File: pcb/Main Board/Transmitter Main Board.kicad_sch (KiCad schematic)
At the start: 16 parts, among them J1 Battery, J10 Neopixel Out, J2 BATTERY MONITOR, J3 i2c, J4 XY JOYSTICK, J5 VR3, J6 Steering, J7 Throttle, J8 UART6/i2c2, J9 UART7, U1 Teensy4.1, U2 TLV73312PDBV, U3 NRF24L01_Breakout

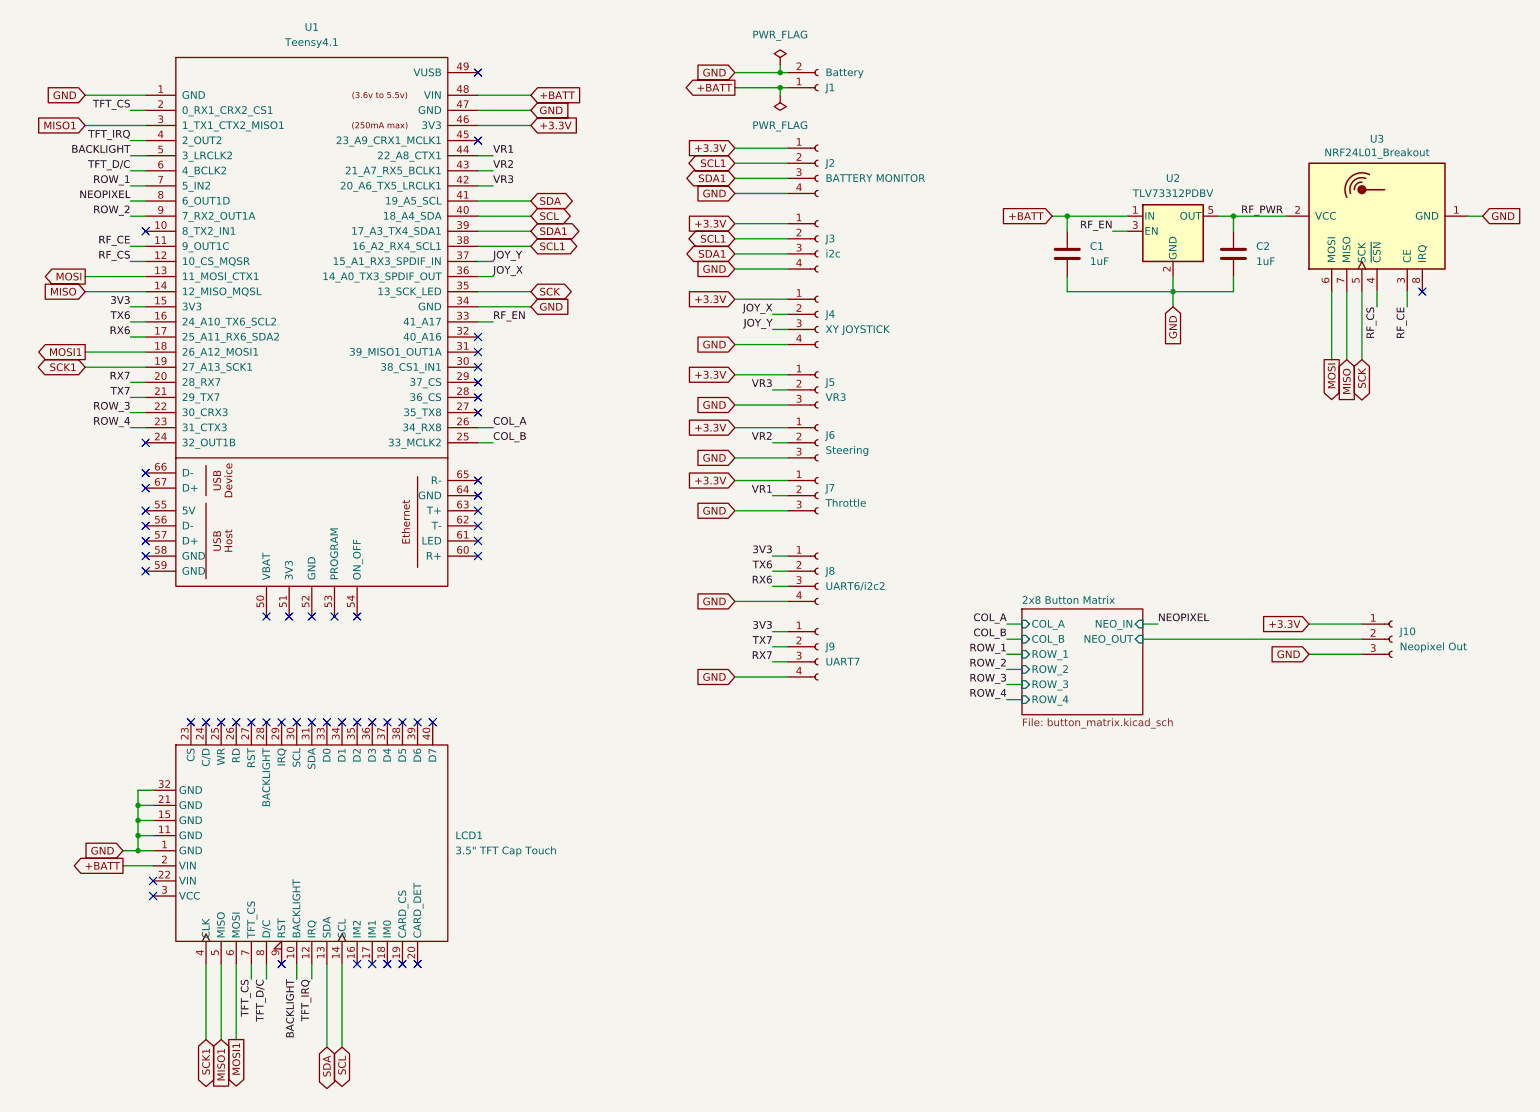
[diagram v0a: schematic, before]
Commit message: Final final routing
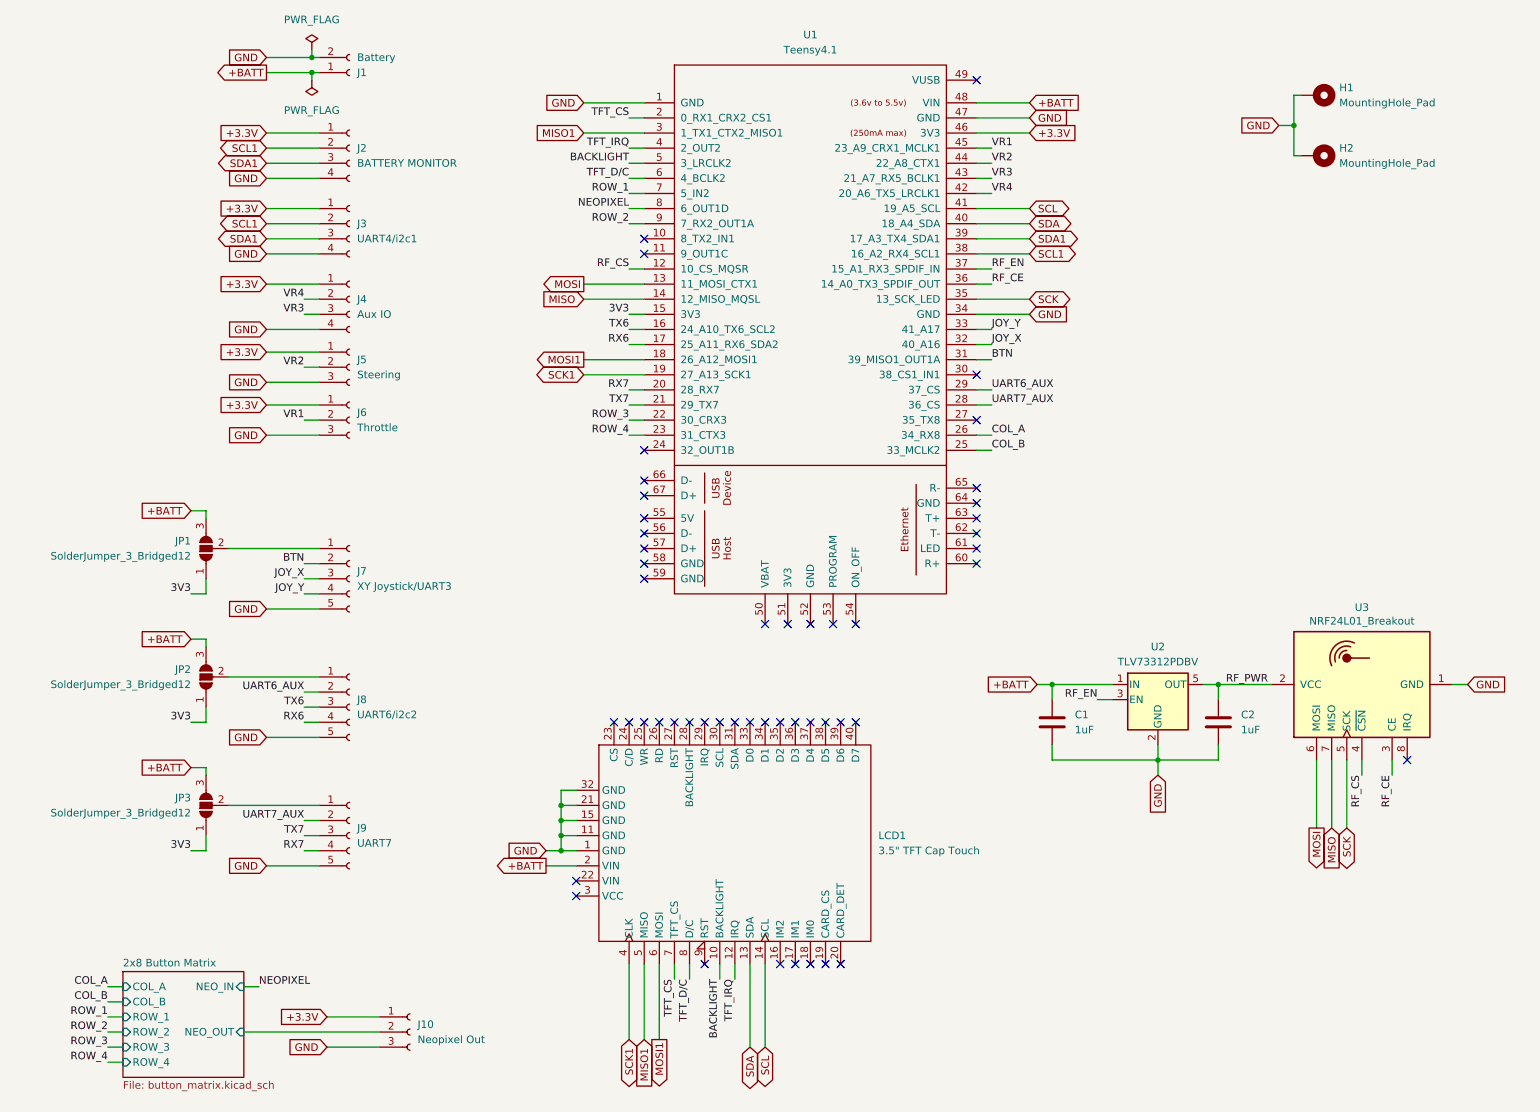
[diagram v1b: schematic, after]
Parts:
- added H1, H2: MountingHole_Pad, MountingHole:MountingHole_3.2mm_M3_Pad, symbol Mechanical:MountingHole_Pad
- added JP1, JP2, JP3: SolderJumper_3_Bridged12, Jumper:SolderJumper-3_P2.0mm_Open_TrianglePad1.0x1.5mm, symbol Jumper:SolderJumper_3_Open
- J3: value i2c -> UART4/i2c1
- J4: renamed from J5; value VR3 -> Aux IO; footprint Connector_JST:JST_PH_B3B-PH-K_1x03_P2.00mm_Vertical -> Connector_JST:JST_PH_B4B-PH-K_1x04_P2.00mm_Vertical; symbol Connector:Conn_01x03_Socket -> Connector:Conn_01x04_Socket
- J7: renamed from J4; value XY JOYSTICK -> XY Joystick/UART3; footprint Connector_JST:JST_PH_B4B-PH-K_1x04_P2.00mm_Vertical -> Connector_JST:JST_PH_B5B-PH-K_1x05_P2.00mm_Vertical; symbol Connector:Conn_01x04_Socket -> Connector:Conn_01x05_Socket
- J8, J9: footprint Connector_JST:JST_PH_B4B-PH-K_1x04_P2.00mm_Vertical -> Connector_JST:JST_PH_B5B-PH-K_1x05_P2.00mm_Vertical; symbol Connector:Conn_01x04_Socket -> Connector:Conn_01x05_Socket
- renumbered J6 to J5, J7 to J6
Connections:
- net +3.3V: no longer J7.1 (Pin_1)
- net +BATT: now also JP1.3 (B), JP2.3 (B), JP3.3 (B)
- net 3V3: now also JP1.1 (A), JP2.1 (A), JP3.1 (A); no longer J8.1 (Pin_1), J9.1 (Pin_1)
- net GND: now also J4.4 (Pin_4), J7.5 (Pin_5), J8.5 (Pin_5), J9.5 (Pin_5), H1.1, H2.1; no longer J4.3 (Pin_3), J7.4 (Pin_4), J8.4 (Pin_4), J9.4 (Pin_4)
- net JOY_X: now also J7.3 (Pin_3), U1.32 (40_A16); no longer J7.2 (Pin_2), U1.36 (14_A0_TX3_SPDIF_OUT)
- net JOY_Y: now also J7.4 (Pin_4), U1.33 (41_A17); no longer J7.3 (Pin_3), U1.37 (15_A1_RX3_SPDIF_IN)
- net RF_CE: now also U1.36 (14_A0_TX3_SPDIF_OUT); no longer U1.11 (9_OUT1C)
- net RF_EN: now also U1.37 (15_A1_RX3_SPDIF_IN); no longer U1.33 (41_A17)
- net RX6: now also J8.4 (Pin_4); no longer J8.3 (Pin_3)
- net RX7: now also J9.4 (Pin_4); no longer J9.3 (Pin_3)
- net SCL: now also U1.41 (19_A5_SCL); no longer U1.40 (18_A4_SDA)
- net SDA: now also U1.40 (18_A4_SDA); no longer U1.41 (19_A5_SCL)
- net TX6: now also J8.3 (Pin_3); no longer J8.2 (Pin_2)
- net TX7: now also J9.3 (Pin_3); no longer J9.2 (Pin_2)
- net VR1: now also U1.45 (23_A9_CRX1_MCLK1); no longer U1.44 (22_A8_CTX1)
- net VR2: now also U1.44 (22_A8_CTX1); no longer U1.43 (21_A7_RX5_BCLK1)
- net VR3: now also J4.3 (Pin_3), U1.43 (21_A7_RX5_BCLK1); no longer J4.2 (Pin_2), U1.42 (20_A6_TX5_LRCLK1)
- net UART7_AUX: now reaches U1.28 (36_CS)
- net UART7_AUX: now also J9.2 (Pin_2)
- net UART6_AUX: now reaches U1.29 (37_CS)
- net UART6_AUX: now also J8.2 (Pin_2)
- net BTN: now reaches U1.31 (39_MISO1_OUT1A)
- net BTN: now also J7.2 (Pin_2)
- new net: J9.1 (Pin_1), JP3.2 (C)
- new net: J8.1 (Pin_1), JP2.2 (C)
- new net: J7.1 (Pin_1), JP1.2 (C)
- new net VR4: J4.2 (Pin_2), U1.42 (20_A6_TX5_LRCLK1)
- no-connect marks 54 -> 50
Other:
- moved on the sheet: C1, C2, J1, J10, J2, J3, J5, J6, LCD1, U1, U2, U3
